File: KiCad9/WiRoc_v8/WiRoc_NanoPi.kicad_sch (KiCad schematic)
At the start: 51 parts, among them J1 Conn_02x05_Odd_Even, J10 Conn_01x09_Socket, J2 Conn_01x04, J5 Conn_01x04_Socket, J6 HAT_Conn_DBG, J8 Conn_01x06, SW1 SW_SPST, U1 SY6280, U10 SY7069ADC, U2 OLED, U3 AXP209, U5 SY6280, U6 BatteryPadM, U7 BatteryPadP

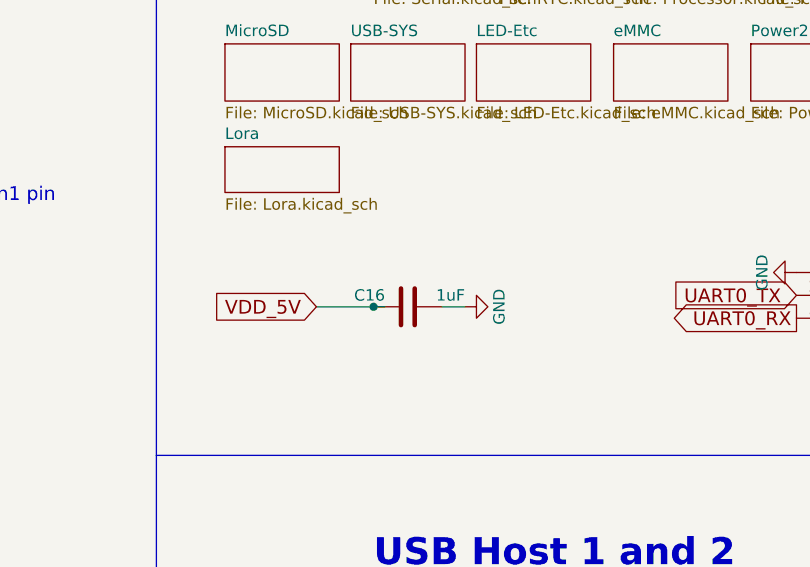
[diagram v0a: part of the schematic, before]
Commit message: etc
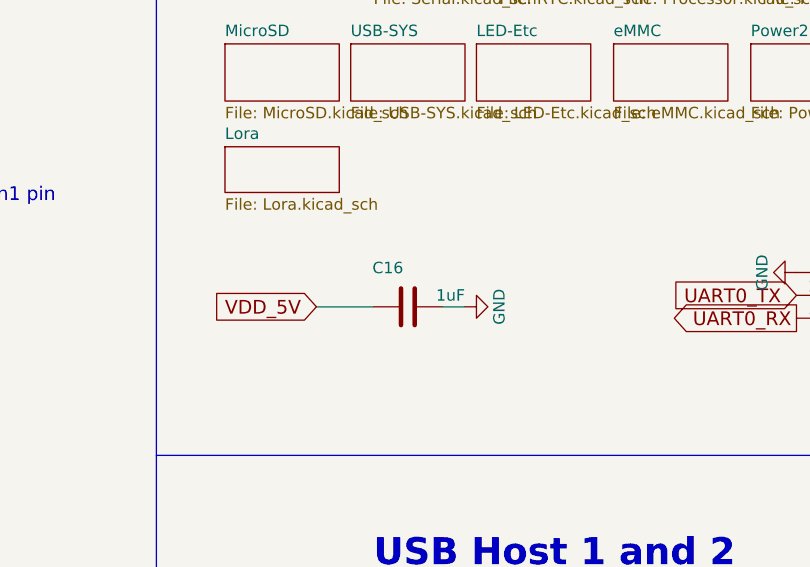
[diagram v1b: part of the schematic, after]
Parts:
- J1, J10, J5: now left out of the parts list
- U1, U5: FT Rotation Offset (none) -> 90; JLCPCB Rotation Offset -90 -> (none)
- U10: FT Rotation Offset (none) -> 0; JLCPCB Rotation Offset 180 -> (none)
